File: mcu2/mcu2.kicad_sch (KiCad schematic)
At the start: 32 parts, among them J1 KF128-5.08, J2 Conn_01x30, J8 Conn_01x30, Q1 WSF3085, Q2 PL4009, Q3 PL4009, U1 Pico, U2 motor_driver, U3 max31865_module, U4 dcdc_module

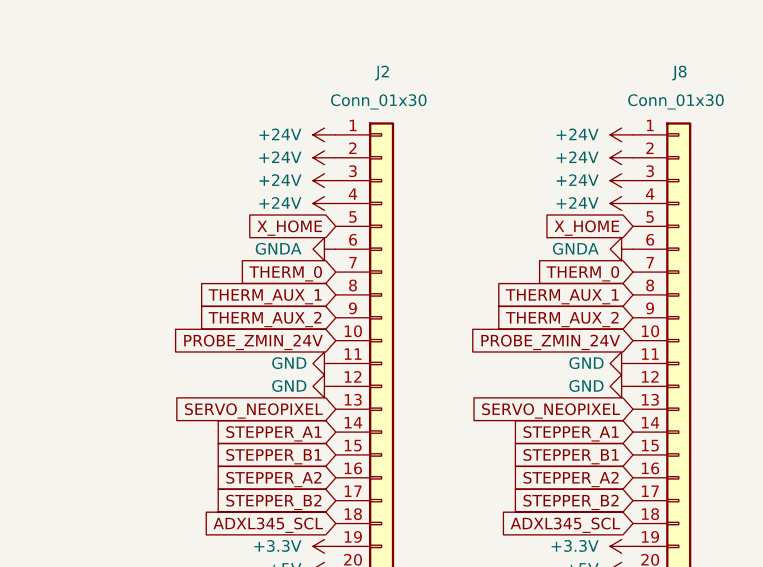
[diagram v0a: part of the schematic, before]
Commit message: mcu2 gerber
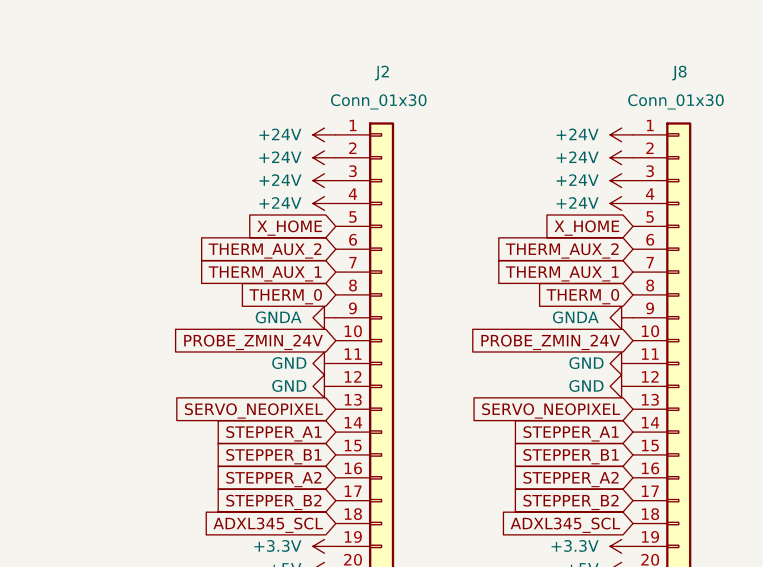
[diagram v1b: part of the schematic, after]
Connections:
- net GNDA: now also J2.9 (Pin_9), J8.9 (Pin_9); no longer J2.6 (Pin_6), J8.6 (Pin_6)
- net THERM_0: now also J2.8 (Pin_8), J8.8 (Pin_8); no longer J2.7 (Pin_7), J8.7 (Pin_7)
- net THERM_AUX_1: now also J2.7 (Pin_7), J8.7 (Pin_7); no longer J2.8 (Pin_8), J8.8 (Pin_8)
- net THERM_AUX_2: now also J2.6 (Pin_6), J8.6 (Pin_6); no longer J2.9 (Pin_9), J8.9 (Pin_9)
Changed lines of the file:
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@@
     )
   )
-  (global_label "THERM_AUX_1" (shape input) (at 240.665 102.87 180) (fields_autoplaced)
-    (effects (font (size 1.27 1.27)) (justify right))
-    (property "Intersheet References" "${INTERSHEET_REFS}" (id 0) (at 225.31 102.7906 0)
+  (global_label "THERM_AUX_1" (shape input) (at 240.665 100.33 180) (fields_autoplaced)
+    (effects (font (size 1.27 1.27)) (justify right))
+    (property "Intersheet References" "${INTERSHEET_REFS}" (id 0) (at 225.31 100.4094 0)
       (effects (font (size 1.27 1.27)) (justify right) hide)
     )
@@
     )
   )
-  (global_label "THERM_AUX_2" (shape input) (at 273.685 105.41 180) (fields_autoplaced)
-    (effects (font (size 1.27 1.27)) (justify right))
-    (property "Intersheet References" "${INTERSHEET_REFS}" (id 0) (at 258.33 105.3306 0)
+  (global_label "THERM_AUX_2" (shape input) (at 273.685 97.79 180) (fields_autoplaced)
+    (effects (font (size 1.27 1.27)) (justify right))
+    (property "Intersheet References" "${INTERSHEET_REFS}" (id 0) (at 258.33 97.8694 0)
       (effects (font (size 1.27 1.27)) (justify right) hide)
     )
@@
     )
   )
-  (global_label "THERM_0" (shape input) (at 273.685 100.33 180) (fields_autoplaced)
-    (effects (font (size 1.27 1.27)) (justify right))
-    (property "Intersheet References" "${INTERSHEET_REFS}" (id 0) (at 262.9262 100.2506 0)
+  (global_label "THERM_0" (shape input) (at 273.685 102.87 180) (fields_autoplaced)
+    (effects (font (size 1.27 1.27)) (justify right))
+    (property "Intersheet References" "${INTERSHEET_REFS}" (id 0) (at 262.9262 102.9494 0)
       (effects (font (size 1.27 1.27)) (justify right) hide)
     )
@@
     )
   )
-  (global_label "THERM_AUX_2" (shape input) (at 240.665 105.41 180) (fields_autoplaced)
-    (effects (font (size 1.27 1.27)) (justify right))
-    (property "Intersheet References" "${INTERSHEET_REFS}" (id 0) (at 225.31 105.3306 0)
+  (global_label "THERM_AUX_2" (shape input) (at 240.665 97.79 180) (fields_autoplaced)
+    (effects (font (size 1.27 1.27)) (justify right))
+    (property "Intersheet References" "${INTERSHEET_REFS}" (id 0) (at 225.31 97.8694 0)
       (effects (font (size 1.27 1.27)) (justify right) hide)
     )
@@
     )
   )
-  (global_label "THERM_0" (shape input) (at 240.665 100.33 180) (fields_autoplaced)
-    (effects (font (size 1.27 1.27)) (justify right))
-    (property "Intersheet References" "${INTERSHEET_REFS}" (id 0) (at 229.9062 100.2506 0)
+  (global_label "THERM_0" (shape input) (at 240.665 102.87 180) (fields_autoplaced)
+    (effects (font (size 1.27 1.27)) (justify right))
+    (property "Intersheet References" "${INTERSHEET_REFS}" (id 0) (at 229.9062 102.9494 0)
       (effects (font (size 1.27 1.27)) (justify right) hide)
     )
@@
     )
   )
-  (global_label "THERM_AUX_1" (shape input) (at 273.685 102.87 180) (fields_autoplaced)
-    (effects (font (size 1.27 1.27)) (justify right))
-    (property "Intersheet References" "${INTERSHEET_REFS}" (id 0) (at 258.33 102.7906 0)
+  (global_label "THERM_AUX_1" (shape input) (at 273.685 100.33 180) (fields_autoplaced)
+    (effects (font (size 1.27 1.27)) (justify right))
+    (property "Intersheet References" "${INTERSHEET_REFS}" (id 0) (at 258.33 100.4094 0)
       (effects (font (size 1.27 1.27)) (justify right) hide)
     )
@@
     (pin "1")
   )
-  (symbol (lib_id "power:GNDA") (at 240.665 97.79 270) (unit 1)
-    (in_bom yes) (on_board yes)
-    (property "Reference" "#PWR037" (id 0) (at 234.315 97.79 0)
-      (effects (font (size 1.27 1.27)) hide)
-    )
-    (property "Value" "GNDA" (id 1) (at 236.855 97.79 90)
-      (effects (font (size 1.27 1.27)) (justify right))
-    )
-    (property "Footprint" "" (id 2) (at 240.665 97.79 0)
-      (effects (font (size 1.27 1.27)) hide)
-    )
-    (property "Datasheet" "" (id 3) (at 240.665 97.79 0)
+  (symbol (lib_id "power:GNDA") (at 240.665 105.41 270) (mirror x) (unit 1)
+    (in_bom yes) (on_board yes)
+    (property "Reference" "#PWR037" (id 0) (at 234.315 105.41 0)
+      (effects (font (size 1.27 1.27)) hide)
+    )
+    (property "Value" "GNDA" (id 1) (at 236.855 105.41 90)
+      (effects (font (size 1.27 1.27)) (justify right))
+    )
+    (property "Footprint" "" (id 2) (at 240.665 105.41 0)
+      (effects (font (size 1.27 1.27)) hide)
+    )
+    (property "Datasheet" "" (id 3) (at 240.665 105.41 0)
       (effects (font (size 1.27 1.27)) hide)
     )
@@
     (pin "2")
   )
-  (symbol (lib_id "power:GNDA") (at 273.685 97.79 270) (unit 1)
-    (in_bom yes) (on_board yes)
-    (property "Reference" "#PWR047" (id 0) (at 267.335 97.79 0)
-      (effects (font (size 1.27 1.27)) hide)
-    )
-    (property "Value" "GNDA" (id 1) (at 269.875 97.79 90)
-      (effects (font (size 1.27 1.27)) (justify right))
-    )
-    (property "Footprint" "" (id 2) (at 273.685 97.79 0)
-      (effects (font (size 1.27 1.27)) hide)
-    )
-    (property "Datasheet" "" (id 3) (at 273.685 97.79 0)
-      (effects (font (size 1.27 1.27)) hide)
-    )
+  (symbol (lib_id "power:GNDA") (at 273.685 105.41 270) (mirror x) (unit 1)
+    (in_bom yes) (on_board yes)
+    (property "Reference" "#PWR047" (id 0) (at 267.335 105.41 0)
+      (effects (font (size 1.27 1.27)) hide)
+    )
+    (property "Value" "GNDA" (id 1) (at 269.875 105.41 90)
+      (effects (font (size 1.27 1.27)) (justify right))
+    )
+    (property "Footprint" "" (id 2) (at 273.685 105.41 0)
+      (effects (font (size 1.27 1.27)) hide)
+    )
+    (property "Datasheet" "" (id 3) (at 273.685 105.41 0)
+      (effects (font (size 1.27 1.27)) hide)
+    )
